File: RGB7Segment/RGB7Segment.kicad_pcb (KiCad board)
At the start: 2 copper layers, 42.5 x 25.5 mm, 20 parts, among them J1 Conn_01x04_Female

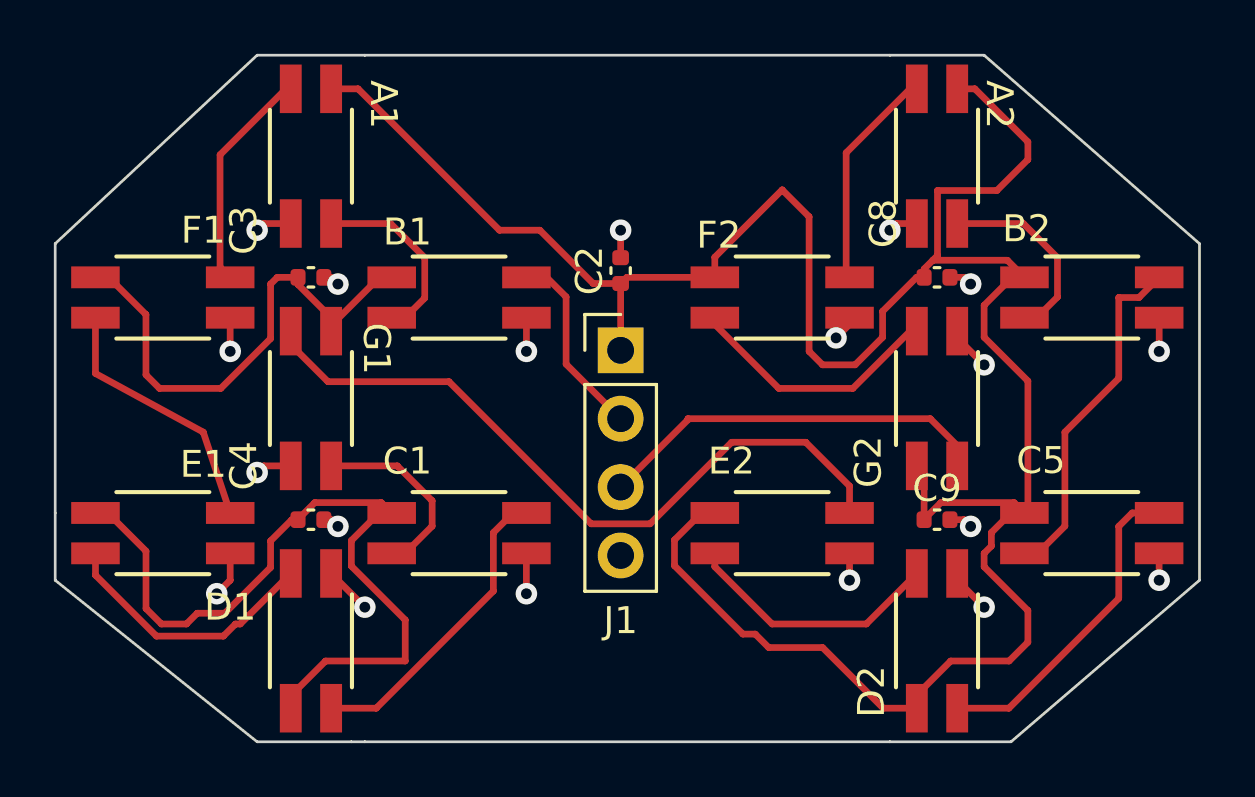
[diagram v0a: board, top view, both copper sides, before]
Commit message: Cleaning up PCB, and minor cleanup.
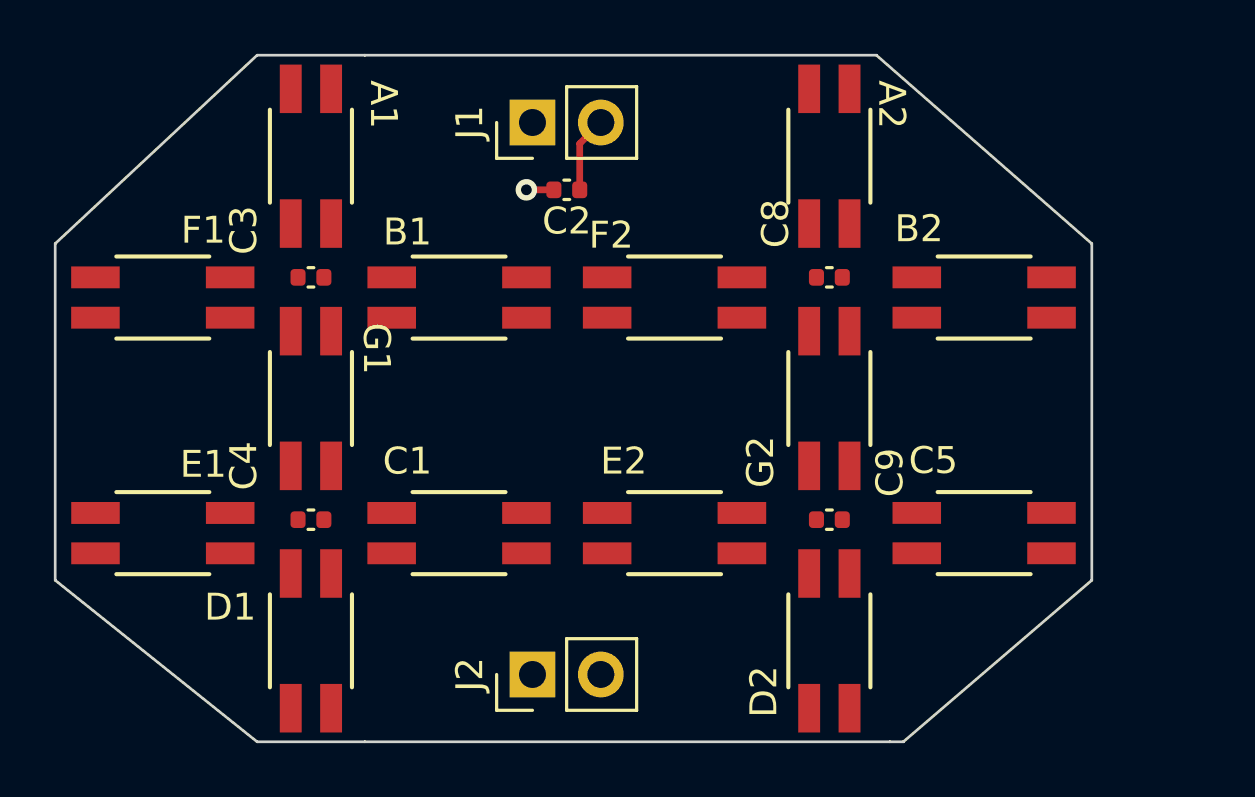
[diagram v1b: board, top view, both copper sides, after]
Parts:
- added J2: Conn_01x02_Socket, Connector_PinHeader_2.54mm:PinHeader_1x02_P2.54mm_Vertical, F.Cu at (207.2, 100.0)
- J1: value Conn_01x04_Female -> Conn_01x02_Socket; footprint Connector_PinHeader_2.54mm:PinHeader_1x04_P2.54mm_Vertical -> Connector_PinHeader_2.54mm:PinHeader_1x02_P2.54mm_Vertical
- moved J1 9.07 mm to (207.2, 79.5), turned to 90 degrees
- moved A2 4.00 mm to (218.3, 80.8)
- moved B2 4.00 mm to (224.0, 86.0)
- moved C5 4.00 mm to (224.0, 94.7)
- moved C8 4.00 mm to (218.3, 85.3)
- moved C9 4.00 mm to (218.3, 94.3)
- moved D2 4.00 mm to (218.3, 98.8)
- moved E2 4.00 mm to (212.5, 94.8)
- moved F2 4.00 mm to (212.5, 86.0)
- moved G2 4.00 mm to (218.3, 89.8)
- moved C2 3.61 mm to (208.5, 82.0), turned to 180 degrees
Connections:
- J1 pad 1: VCC -> GND
- J1 pad 2: /DIN -> VCC
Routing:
- net VCC: track 142.6 -> 3.70 mm
- net /E2: track 26.9 -> 0.00 mm
- net GND: track 22.8 -> 1.02 mm, vias 19 -> 1
- net /DOUT: track 14.7 -> 0.00 mm
- net /B2: track 13.1 -> 0.00 mm
- net /C2: track 12.1 -> 0.00 mm
- net /C1: track 11.5 -> 0.00 mm
- net /D1: track 9.97 -> 0.00 mm
- net /E1: track 9.79 -> 0.00 mm
- net /D2: track 9.66 -> 0.00 mm
- net /G2: track 9.62 -> 0.00 mm
- net /F1: track 8.35 -> 0.00 mm
- net /F2: track 8.29 -> 0.00 mm
- net /A2: track 7.26 -> 0.00 mm
- net /G1: track 7.15 -> 0.00 mm
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- added copper zone on B.Cu, net GND
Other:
- board size 42.5 x 25.5 mm -> 38.5 x 25.5 mm
